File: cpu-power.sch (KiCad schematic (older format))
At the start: 3 parts

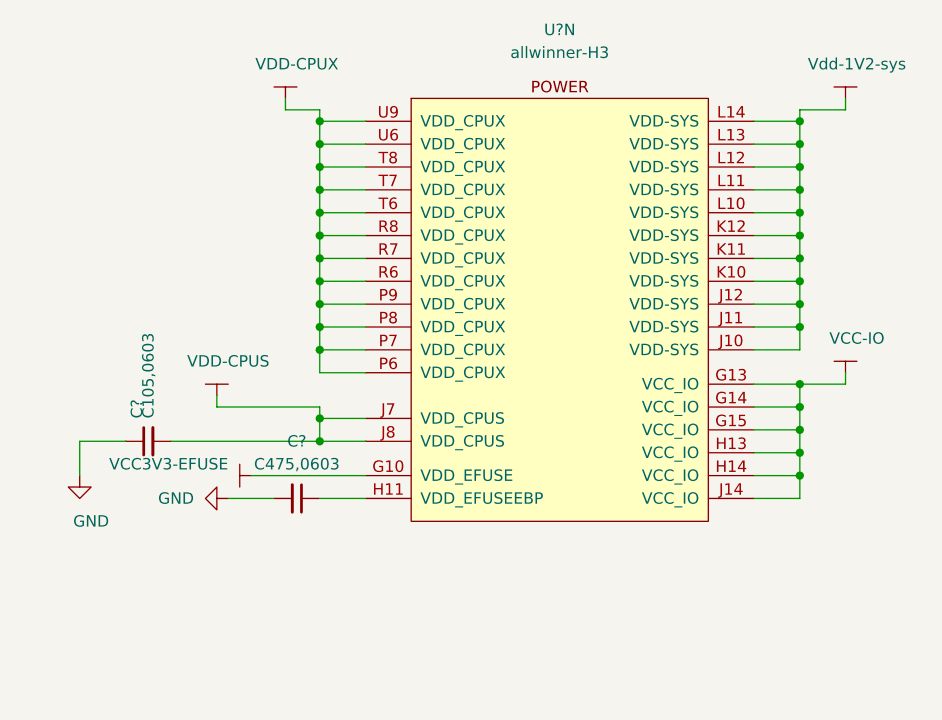
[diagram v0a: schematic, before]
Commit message: update,
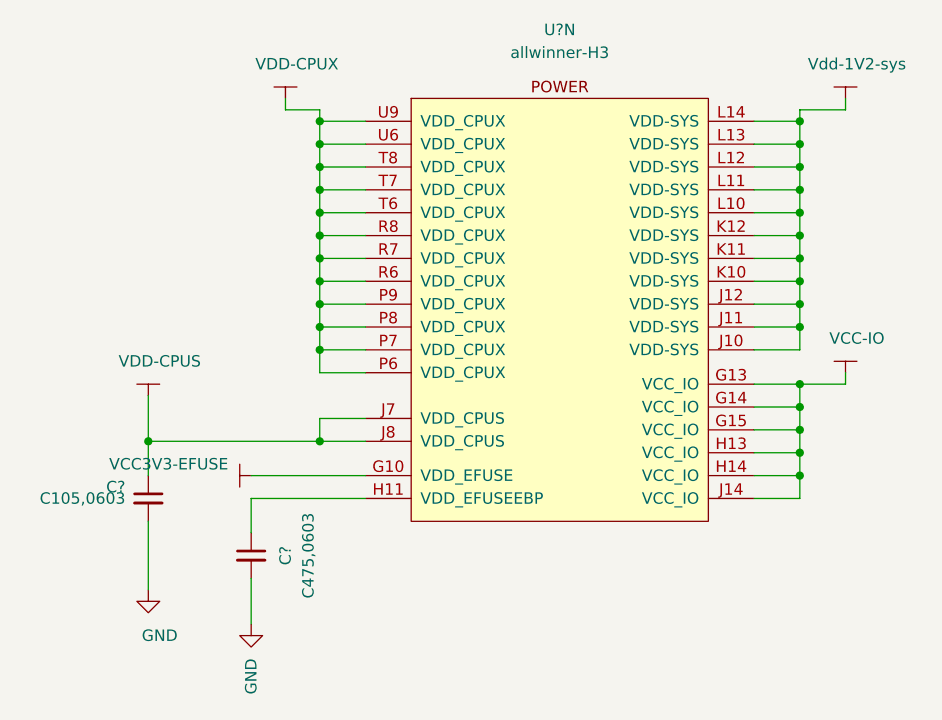
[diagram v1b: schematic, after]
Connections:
- net GND: now also C?.2; no longer C?.1
- net VDD-CPUS: now also C?.1; no longer C?.2
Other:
- moved on the sheet: C?
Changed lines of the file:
@@
 L taobao-components:VDD-CPUS #PWR?
 U 1 1 5C6598C1
-P 6650 6450
+P 6350 6450
 AR Path="/5C5C55F2/5C6598C1" Ref="#PWR?"  Part="1"
 AR Path="/5C660882/5C6598C1" Ref="#PWR?"  Part="1"
 AR Path="/5C273FE9/5C291027/5C6598C1" Ref="#PWR?"  Part="1"
 AR Path="/5C7B767A/5C291027/5C6598C1" Ref="#PWR?"  Part="1"
-F 0 "#PWR?" H 6650 6300 50  0001 C CNN
-F 1 "VDD-CPUS" H 6700 6600 50  0000 C CNN
-F 2 "" H 6650 6450 50  0001 C CNN
-F 3 "" H 6650 6450 50  0001 C CNN
-	1    6650 6450
+F 0 "#PWR?" H 6350 6300 50  0001 C CNN
+F 1 "VDD-CPUS" H 6400 6600 50  0000 C CNN
+F 2 "" H 6350 6450 50  0001 C CNN
+F 3 "" H 6350 6450 50  0001 C CNN
+	1    6350 6450
 	1    0    0    -1
 $EndComp
 Wire Wire Line
-	6650 6450 6650 6500
-Wire Wire Line
-	6650 6500 7100 6500
-Wire Wire Line
-	7100 6500 7100 6550
-Wire Wire Line
 	7100 6650 7300 6650
 Wire Wire Line
 	7300 6550 7100 6550
-Connection ~ 7100 6550
 Wire Wire Line
 	7100 6550 7100 6650
@@
 L taobao-c:C105,0603 C?
 U 1 1 5C65C4E7
-P 6350 6650
+P 6350 6900
 AR Path="/5C5C55F2/5C65C4E7" Ref="C?"  Part="1"
 AR Path="/5C660882/5C65C4E7" Ref="C?"  Part="1"
 AR Path="/5C273FE9/5C291027/5C65C4E7" Ref="C?"  Part="1"
 AR Path="/5C7B767A/5C291027/5C65C4E7" Ref="C?"  Part="1"
-F 0 "C?" H 6450 6700 50  0000 L CNN
-F 1 "C105,0603" H 6450 6650 50  0000 L CNN
-F 2 "Capacitor_SMD:C_0603_1608Metric_Pad1.05x0.95mm_HandSolder" H 6350 6650 50  0001 C CNN
-F 3 "~" H 6350 6650 50  0001 C CNN
-	1    6350 6650
-	0    -1   -1   0
+F 0 "C?" H 6250 6950 50  0000 R CNN
+F 1 "C105,0603" H 6250 6900 50  0000 R CNN
+F 2 "Capacitor_SMD:C_0603_1608Metric_Pad1.05x0.95mm_HandSolder" H 6350 6900 50  0001 C CNN
+F 3 "~" H 6350 6900 50  0001 C CNN
+	1    6350 6900
+	1    0    0    -1
 $EndComp
 Connection ~ 7100 6650
@@
 L power:GND #PWR?
 U 1 1 5C65DD66
-P 6050 6800
+P 6350 7300
 AR Path="/5C5C55F2/5C65DD66" Ref="#PWR?"  Part="1"
 AR Path="/5C660882/5C65DD66" Ref="#PWR?"  Part="1"
 AR Path="/5C273FE9/5C291027/5C65DD66" Ref="#PWR?"  Part="1"
 AR Path="/5C7B767A/5C291027/5C65DD66" Ref="#PWR?"  Part="1"
-F 0 "#PWR?" H 6050 6550 50  0001 C CNN
-F 1 "GND" H 6100 6600 50  0000 C CNN
-F 2 "" H 6050 6800 50  0001 C CNN
-F 3 "" H 6050 6800 50  0001 C CNN
-	1    6050 6800
+F 0 "#PWR?" H 6350 7050 50  0001 C CNN
+F 1 "GND" H 6400 7100 50  0000 C CNN
+F 2 "" H 6350 7300 50  0001 C CNN
+F 3 "" H 6350 7300 50  0001 C CNN
+	1    6350 7300
 	1    0    0    -1
 $EndComp
-Wire Wire Line
-	6050 6800 6050 6650
 $Bitmap
 Pos 7950 3200
@@
 	0    -1   -1   0
 $EndComp
-Wire Wire Line
-	6450 6650 7100 6650
-Wire Wire Line
-	6250 6650 6050 6650
 $Comp
 L taobao-c:C475,0603 C?
 U 1 1 5C2FD674
-P 7000 6900
-F 0 "C?" V 6750 6900 50  0000 C CNN
-F 1 "C475,0603" V 6850 6900 50  0000 C CNN
-F 2 "Capacitor_SMD:C_0603_1608Metric_Pad1.05x0.95mm_HandSolder" H 7000 6900 50  0001 C CNN
-F 3 "~" H 7000 6900 50  0001 C CNN
-	1    7000 6900
-	0    1    1    0
+P 6800 7150
+F 0 "C?" V 6950 7150 50  0000 C CNN
+F 1 "C475,0603" V 7050 7150 50  0000 C CNN
+F 2 "Capacitor_SMD:C_0603_1608Metric_Pad1.05x0.95mm_HandSolder" H 6800 7150 50  0001 C CNN
+F 3 "~" H 6800 7150 50  0001 C CNN
+	1    6800 7150
+	1    0    0    -1
 $EndComp
 $Comp
 L power:GND #PWR?
 U 1 1 5C2FD702
-P 6700 6900
-F 0 "#PWR?" H 6700 6650 50  0001 C CNN
-F 1 "GND" V 6700 6750 50  0000 R CNN
-F 2 "" H 6700 6900 50  0001 C CNN
-F 3 "" H 6700 6900 50  0001 C CNN
-	1    6700 6900
-	0    1    1    0
+P 6800 7450
+F 0 "#PWR?" H 6800 7200 50  0001 C CNN
+F 1 "GND" V 6800 7300 50  0000 R CNN
+F 2 "" H 6800 7450 50  0001 C CNN
+F 3 "" H 6800 7450 50  0001 C CNN
+	1    6800 7450
+	1    0    0    -1
 $EndComp
 Wire Wire Line
-	6700 6900 6900 6900
-Wire Wire Line
-	7100 6900 7300 6900
+	6800 7450 6800 7250
 Wire Wire Line
 	6800 6800 7300 6800
+Wire Wire Line
+	6800 7050 6800 6900
+Wire Wire Line
+	6800 6900 7300 6900
+Wire Wire Line
+	6350 7000 6350 7300
+Wire Wire Line
+	6350 6800 6350 6650
+Wire Wire Line
+	6350 6650 7100 6650
+Wire Wire Line
+	6350 6450 6350 6650
+Connection ~ 6350 6650
 $EndSCHEMATC
